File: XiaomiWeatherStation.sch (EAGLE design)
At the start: 8 parts

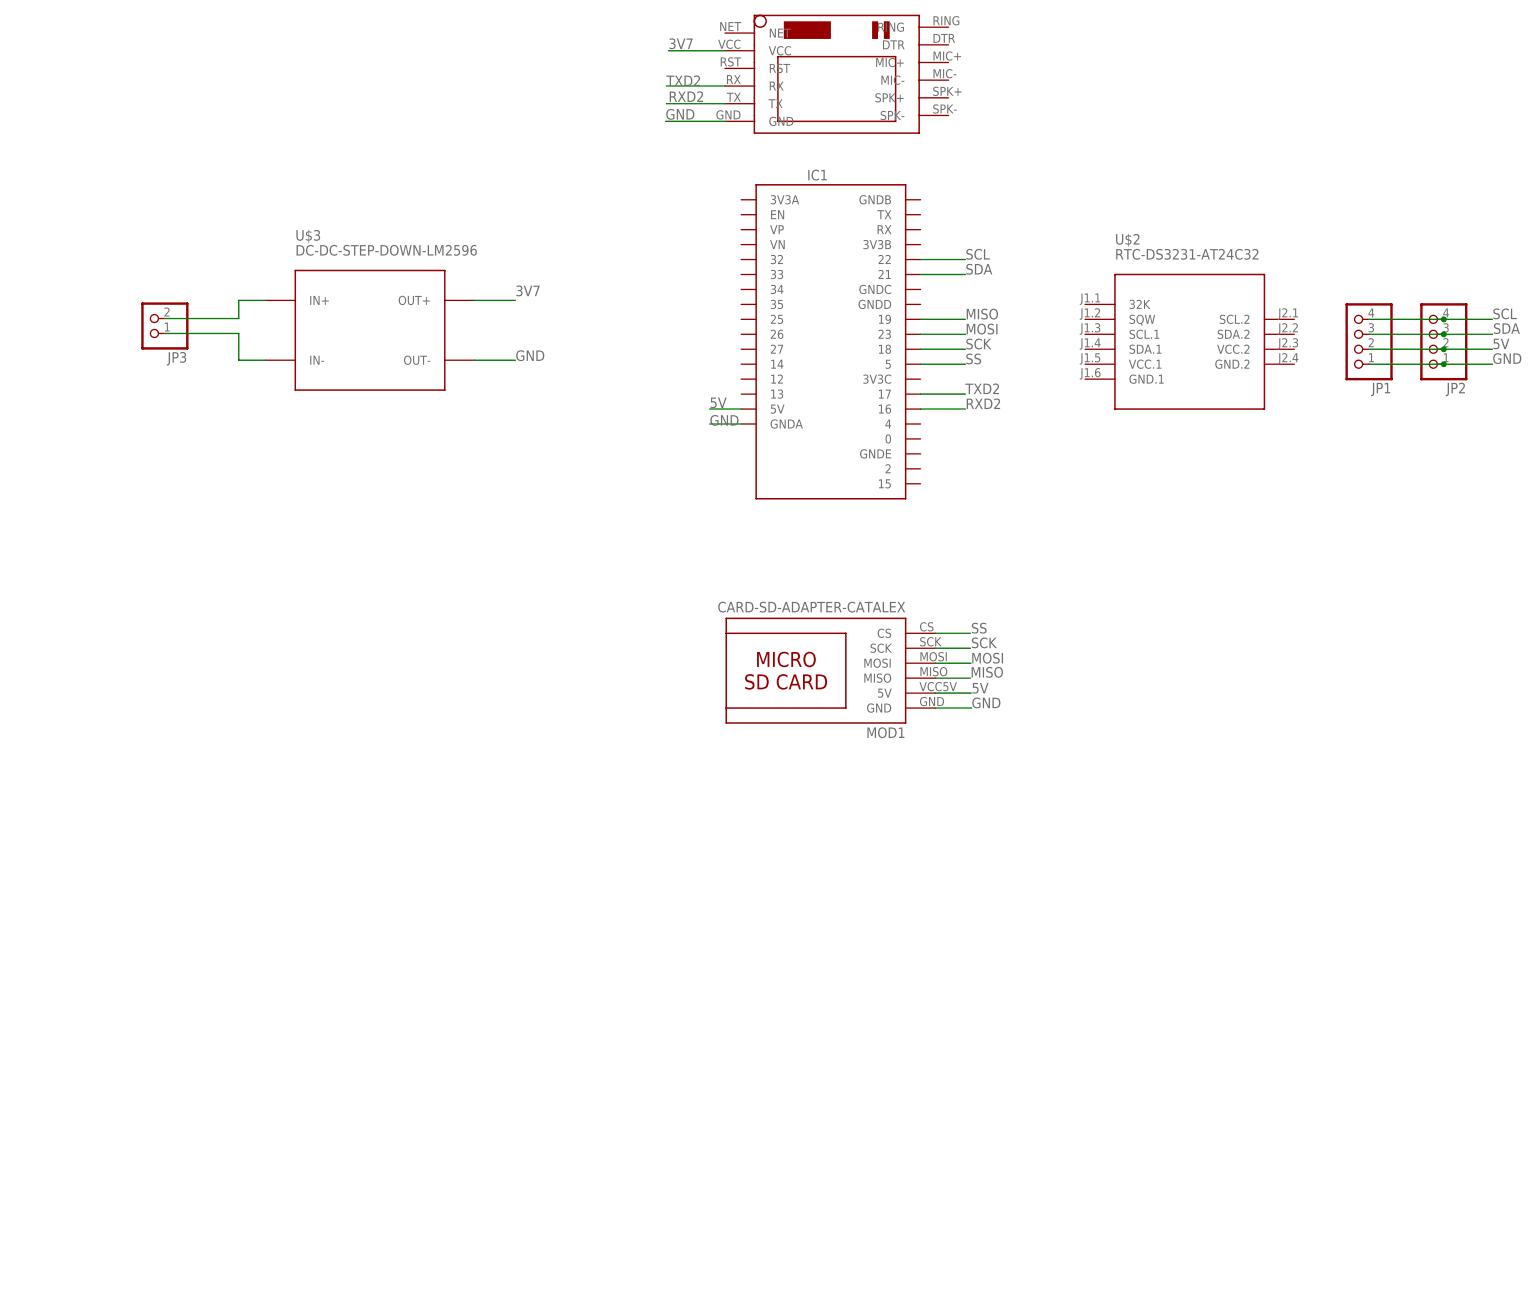
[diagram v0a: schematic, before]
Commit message: Finish routing
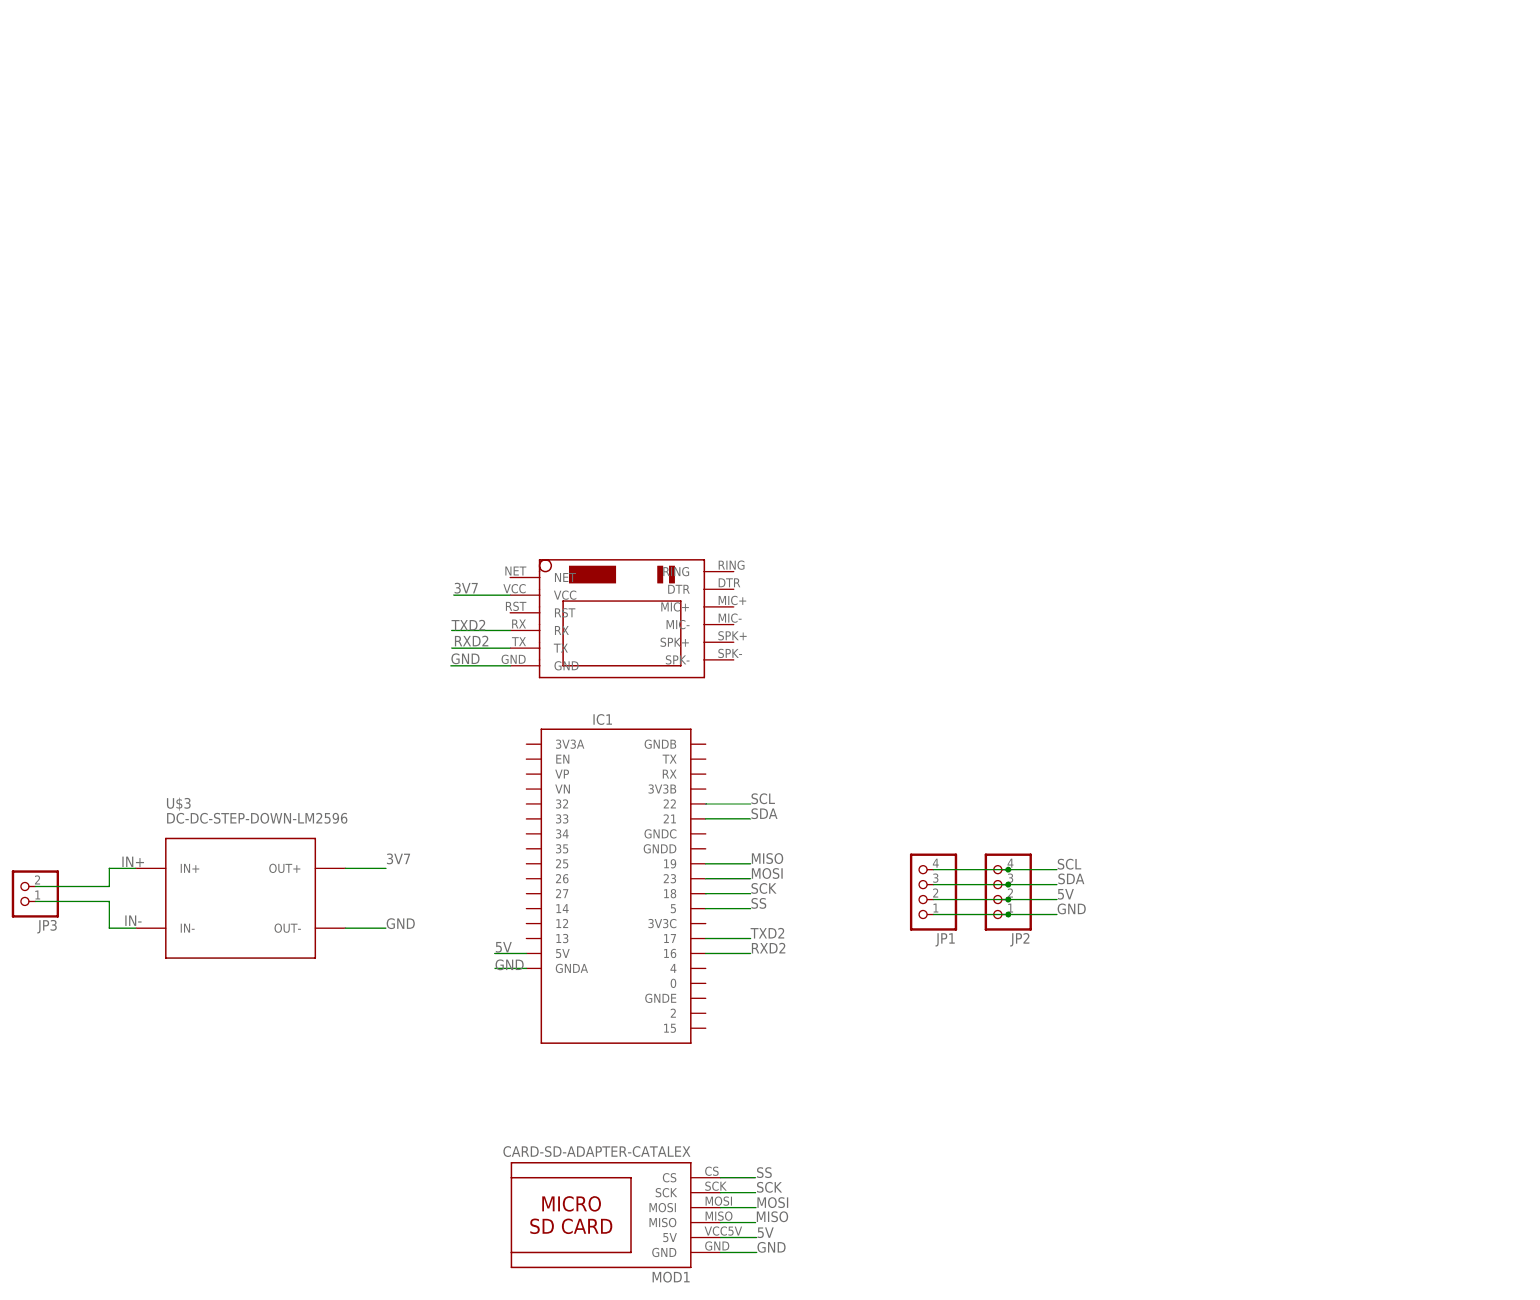
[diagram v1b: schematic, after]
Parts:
- removed U$2: RTC-DS3231-AT24C32, diy-modules:RTC-DS3231-AT24C32
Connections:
- net N$1 renamed IN+
- net N$2 renamed IN-
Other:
- moved on the sheet: IC1, JP1, JP2, JP3, MOD1, U$3
